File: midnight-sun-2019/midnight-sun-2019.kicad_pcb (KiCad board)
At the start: 4 copper layers, 223.5 x 156.2 mm, 551 parts, among them J1 Conn_02x02_Odd_Even, J2 USB_B_Micro, SW1 SW_SPDT, SW2 SW_SPDT, SW3 SW_SPDT, U1 74HC14, U10 74HC14, U11 74HC86, U12 74HC86, U13 74HC86, U14 74HC86, U15 74HC14, U16 74HC14, U2 74HC595, U3 74HC595, U4 74HC595, U5 74HC86, U6 74HC86, U7 74HC86, U8 74HC86, U9 74HC14

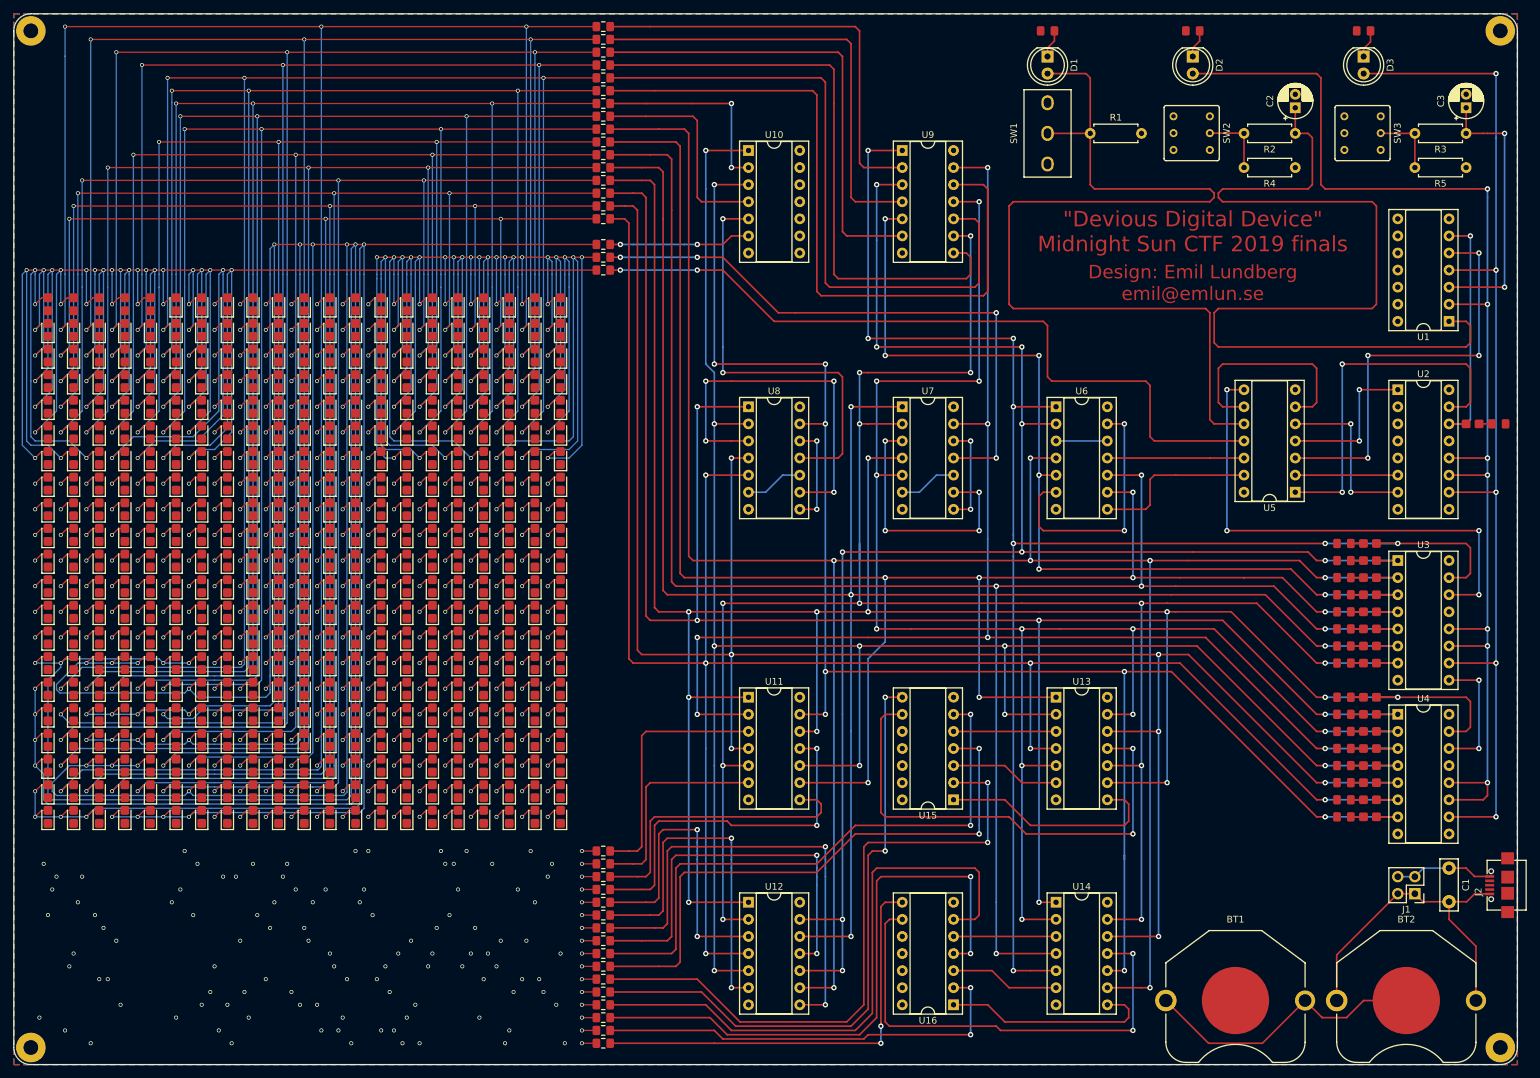
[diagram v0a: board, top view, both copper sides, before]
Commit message: More finishing touches
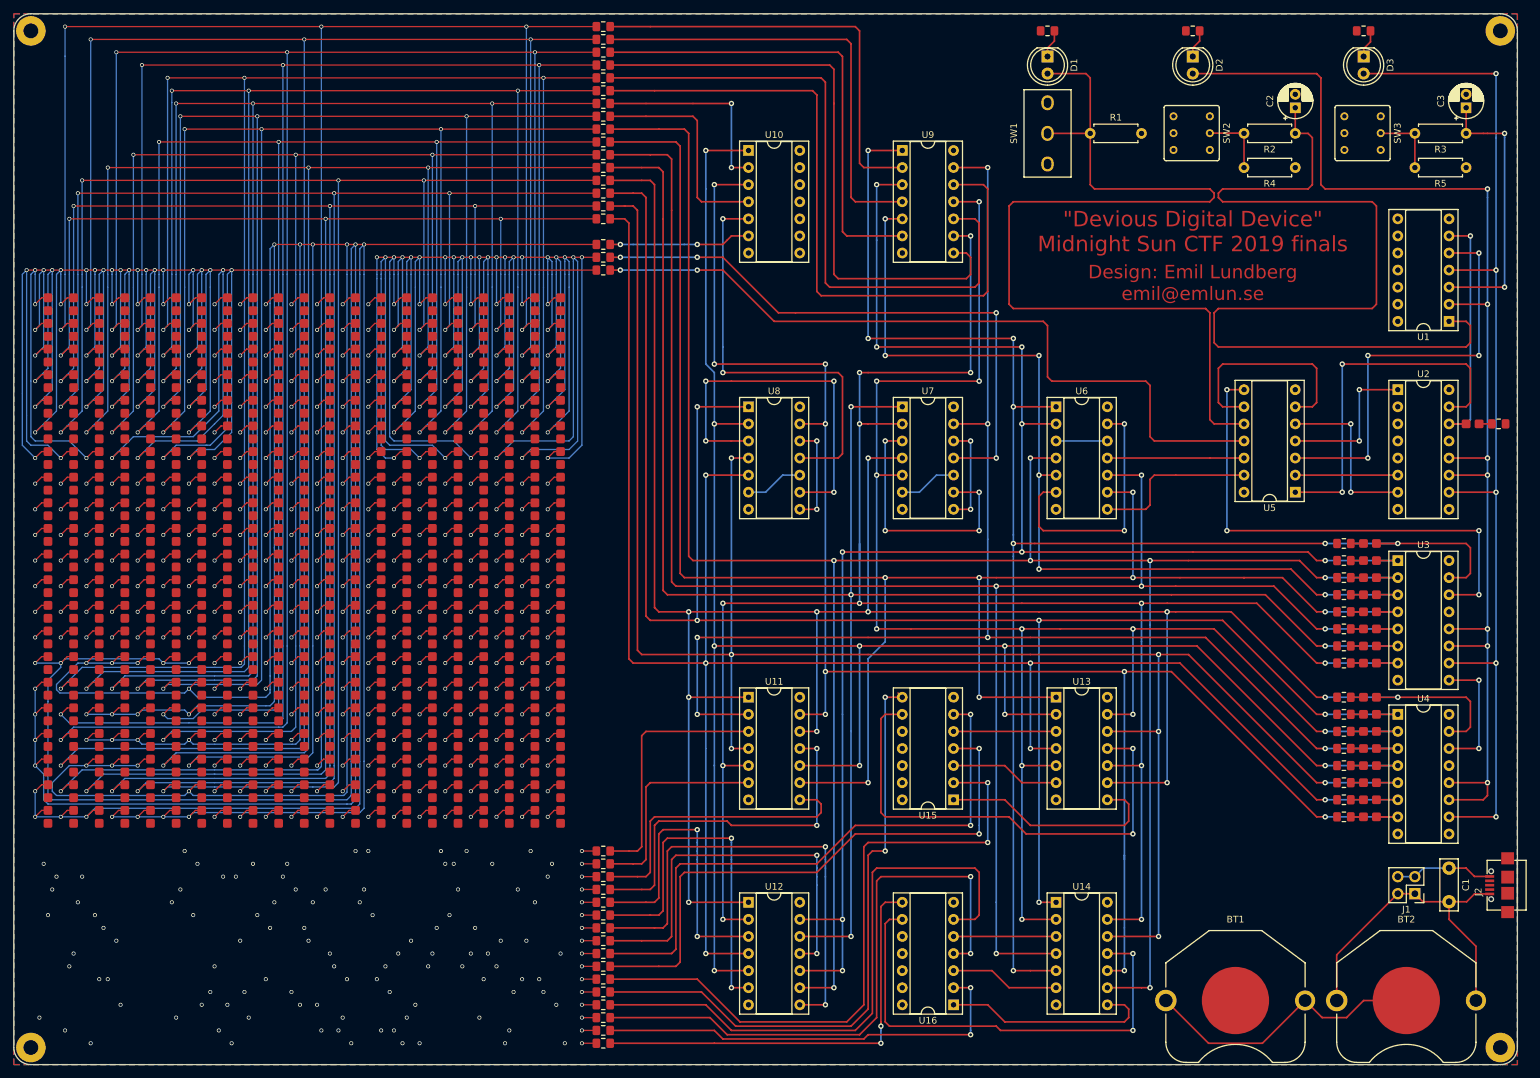
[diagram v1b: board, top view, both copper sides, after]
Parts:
- D100, D101, D102, D103, D104, D105, D106, D107, D108, D109, D110, D111, D112, D113, D114, D115, D116, D117, D118, D119, D120, D121, D122, D123, D124, D125, D126, D127, D128, D129, D130, D131, D132, D133, D134, D135, D136, D137, D138, D139, D140, D141, D142, D143, D144, D145, D146, D147, D148, D149, D150, D151, D152, D153, D154, D155, D156, D157, D158, D159, D160, D161, D162, D163, D164, D165, D166, D167, D168, D169, D170, D171, D172, D173, D174, D175, D176, D177, D178, D179, D180, D181, D182, D183, D184, D185, D186, D187, D188, D189, D190, D191, D192, D193, D194, D195, D196, D197, D198, D199, D200, D201, D202, D203, D204, D205, D206, D207, D208, D209, D210, D211, D212, D213, D214, D215, D216, D217, D218, D219, D220, D221, D222, D223, D224, D225, D226, D227, D228, D229, D230, D231, D232, D233, D234, D235, D236, D237, D238, D239, D240, D241, D242, D243, D244, D245, D246, D247, D248, D249, D250, D251, D252, D253, D254, D255, D256, D257, D258, D259, D26, D260, D261, D262, D263, D264, D265, D266, D267, D268, D269, D27, D270, D271, D272, D273, D274, D275, D276, D277, D278, D279, D28, D280, D281, D282, D283, D284, D285, D286, D287, D288, D289, D29, D290, D291, D292, D293, D294, D295, D296, D297, D298, D299, D30, D300, D301, D302, D303, D304, D305, D306, D307, D308, D309, D31, D310, D311, D312, D313, D314, D315, D316, D317, D318, D319, D32, D320, D321, D322, D323, D324, D325, D326, D327, D328, D329, D33, D330, D331, D332, D333, D334, D335, D336, D337, D338, D339, D34, D340, D341, D342, D343, D344, D345, D346, D347, D348, D349, D35, D350, D351, D352, D353, D354, D355, D356, D357, D358, D359, D36, D360, D361, D362, D363, D364, D365, D366, D367, D368, D369, D37, D370, D371, D372, D373, D374, D375, D376, D377, D378, D379, D38, D380, D381, D382, D383, D384, D385, D386, D387, D388, D389, D39, D390, D391, D392, D393, D394, D395, D396, D397, D398, D399, D40, D400, D401, D402, D403, D404, D405, D406, D407, D408, D409, D41, D410, D411, D412, D413, D414, D415, D416, D417, D418, D419, D42, D420, D421, D422, D423, D424, D425, D426, D427, D428, D429, D43, D430, D431, D432, D433, D434, D435, D436, D437, D438, D439, D44, D440, D441, D442, D443, D444, D445, D446, D447, D448, D449, D45, D450, D451, D452, D453, D454, D455, D456, D457, D458, D459, D46, D460, D461, D47, D48, D49, D50, D51, D52, D53, D54, D55, D56, D57, D58, D59, D60, D61, D62, D63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: footprint LED_SMD:LED_0805_2012Metric_Castellated -> electrokit:LED_0805_2012Metric_Castellated_no_silkscreen
